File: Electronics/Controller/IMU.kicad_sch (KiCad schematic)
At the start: 9 parts, among them J10 CAN BUS, J9 TERM, U5 TJA1462ATK-0Z, U6 PESD2CANFD24V-TR

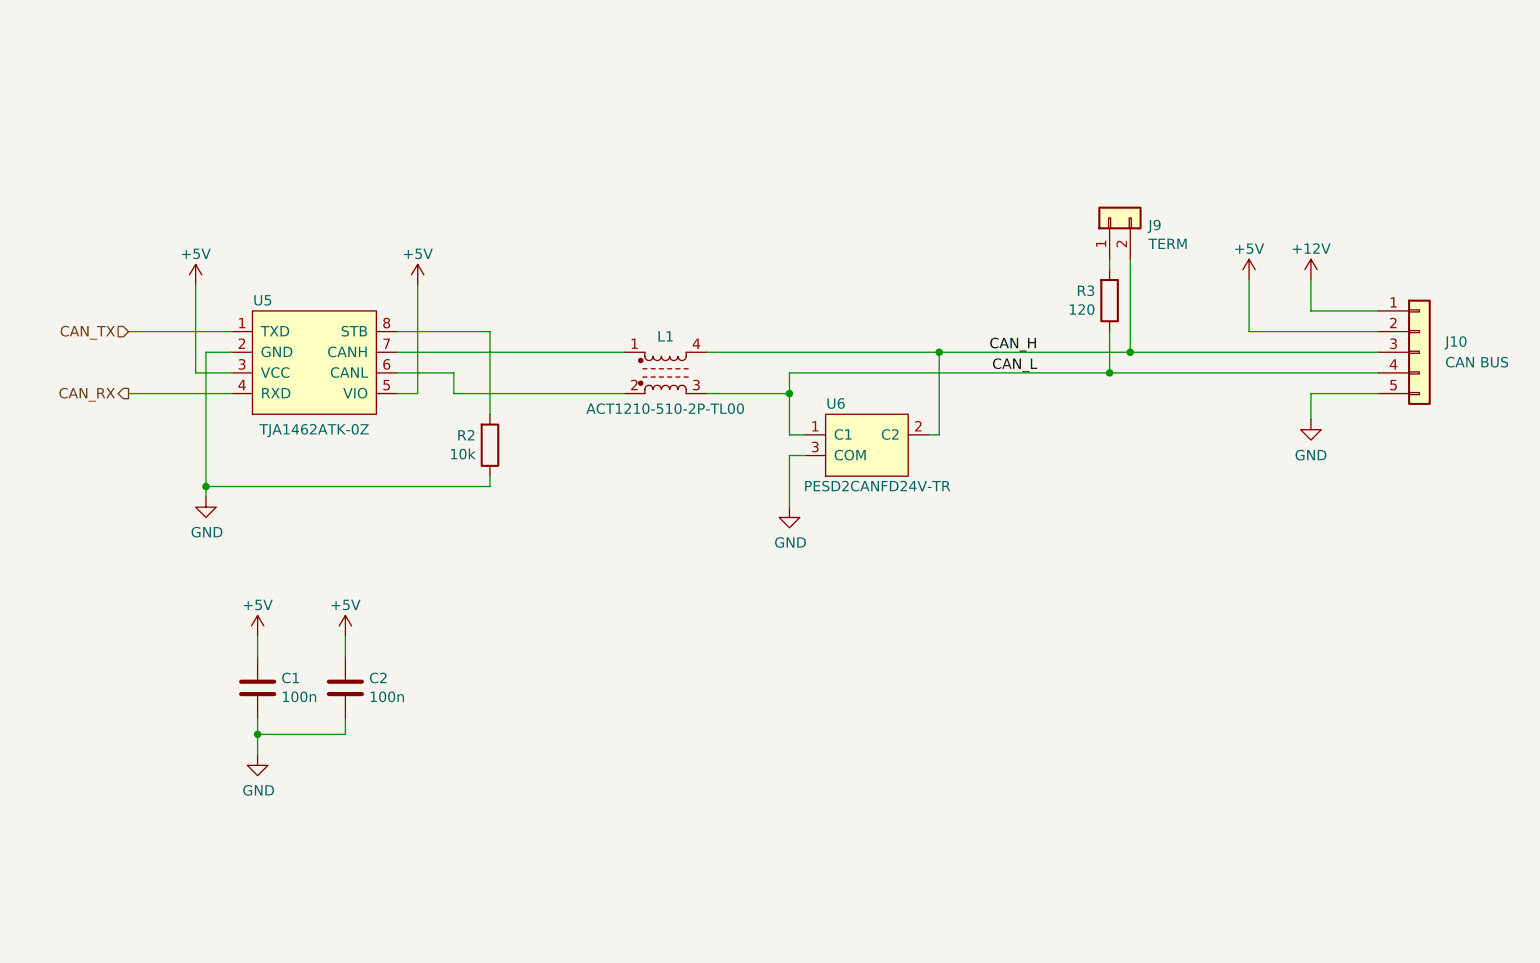
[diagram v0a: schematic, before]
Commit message: Working on PCB layout.
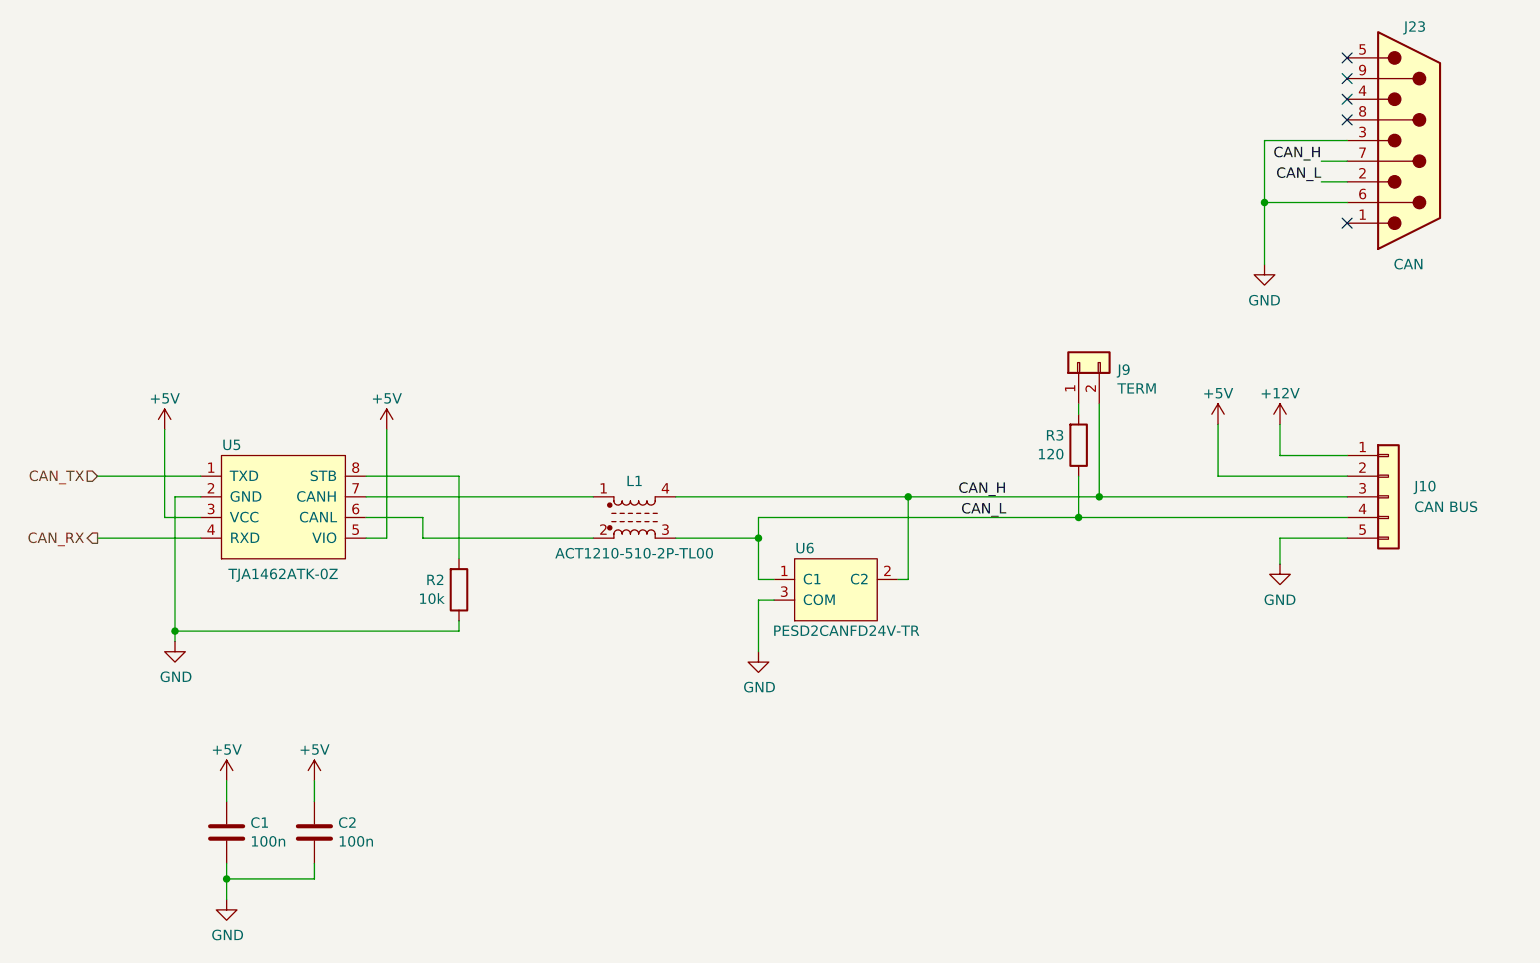
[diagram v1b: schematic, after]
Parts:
- added J23: CAN, EmSA:DB9_RA_MALE_LD09P13A4, symbol Connector:DB9_Male
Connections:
- net CAN_H: now also J23.7
- net CAN_L: now also J23.2
- net GND: now also J23.3, J23.6
- no-connect marks 0 -> 5
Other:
- moved on the sheet: C1, C2, J10, J9, L1, R2, R3, U5, U6
